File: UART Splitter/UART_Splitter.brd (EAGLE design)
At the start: 40.6 x 24.1 mm, 31 parts, among them IC1 ATTINY10, Q1 12mhz, U1 74HC4052

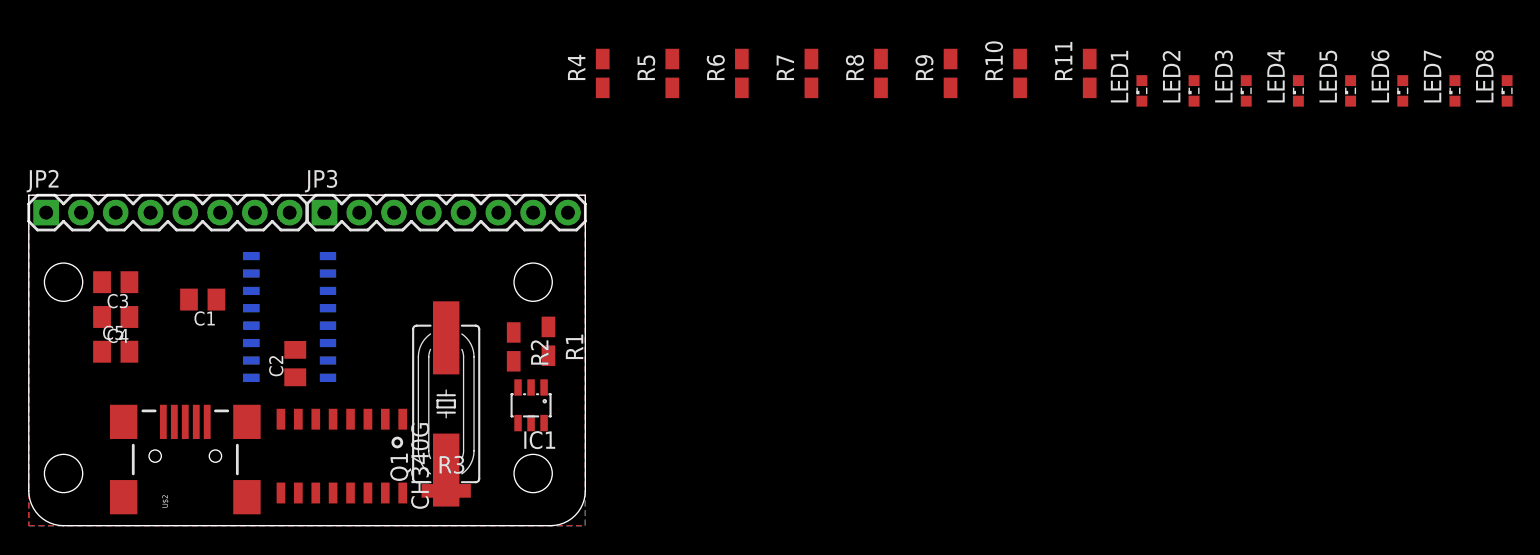
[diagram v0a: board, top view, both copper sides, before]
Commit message: UART Splitter
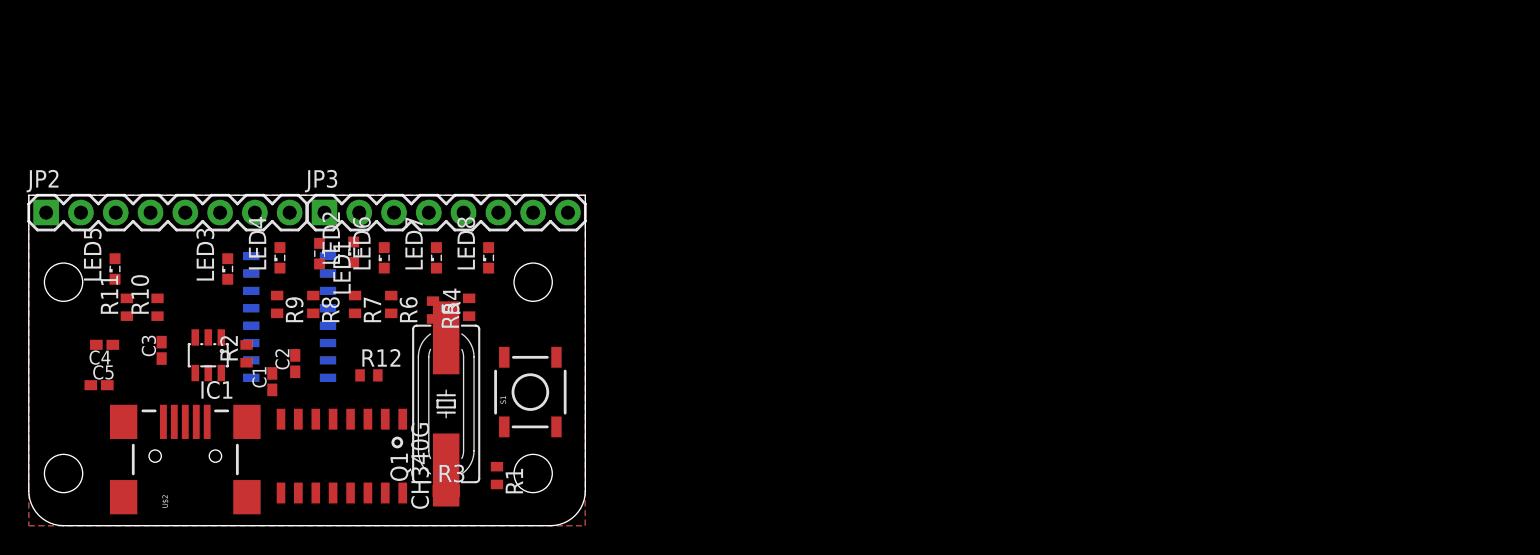
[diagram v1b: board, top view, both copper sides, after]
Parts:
- added R12: 10k, resistor:R0402
- added S1: (no value), SparkFun-Electromechanical:TACTILE_SWITCH_SMD
- C1, C2, C3, C4, C5: device resistor:C0805K -> resistor:C0402K
- R1, R10, R11, R2, R3, R4, R5, R6, R7, R8, R9: device resistor:R0805W -> resistor:R0402
- moved LED5 91.2 mm to (35.5, 18.7)
- moved LED3 75.5 mm to (43.7, 18.7)
- moved LED4 75.4 mm to (47.5, 19.6)
- moved LED6 75.4 mm to (55.2, 19.6)
- moved LED7 75.4 mm to (59.0, 19.6)
- moved LED8 75.4 mm to (62.8, 19.6)
- moved R11 72.3 mm to (36.4, 16.0)
- moved R10 65.3 mm to (38.6, 16.0)
- moved LED2 62.5 mm to (52.9, 20.0)
- moved LED1 61.2 mm to (50.4, 19.9), turned to 270 degrees
- moved R9 52.0 mm to (47.3, 16.2), turned to 270 degrees
- moved R8 44.8 mm to (50.0, 16.2), turned to 270 degrees
- moved R7 37.3 mm to (53.0, 16.2), turned to 270 degrees
- moved R6 30.7 mm to (55.7, 16.2), turned to 270 degrees
- moved R5 24.6 mm to (58.7, 15.7), turned to 270 degrees
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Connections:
- new net N$13: R12.1, U1.6
- net GND: now also S1.3, S1.4
- net N$2: now also R1.2
- net N$6: no longer R1.1
- net N$7: now also IC1.3, R1.1, S1.1, S1.2; no longer U1.6
- net N$8: now also IC1.6, R12.2; no longer IC1.1, R1.2
- net N$9: now also IC1.1; no longer IC1.3

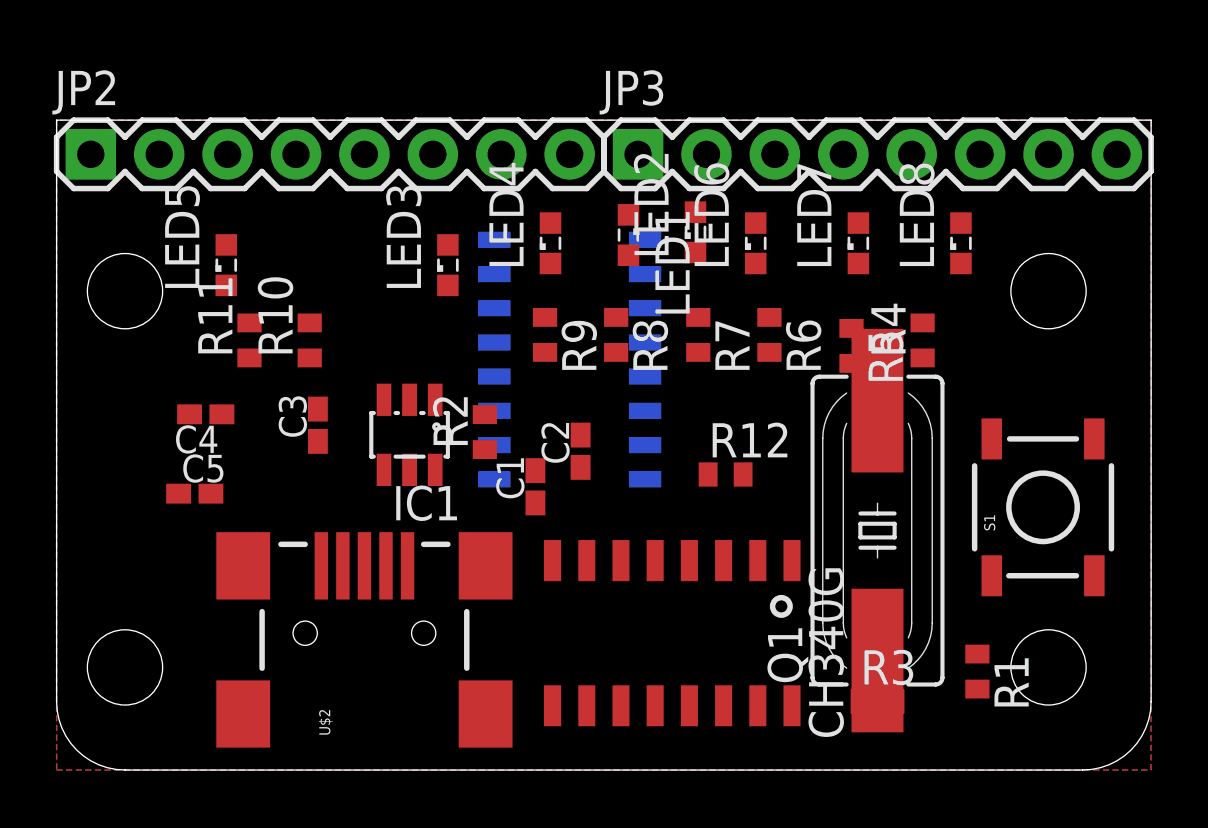
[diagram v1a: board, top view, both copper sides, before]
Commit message: UART Splitter
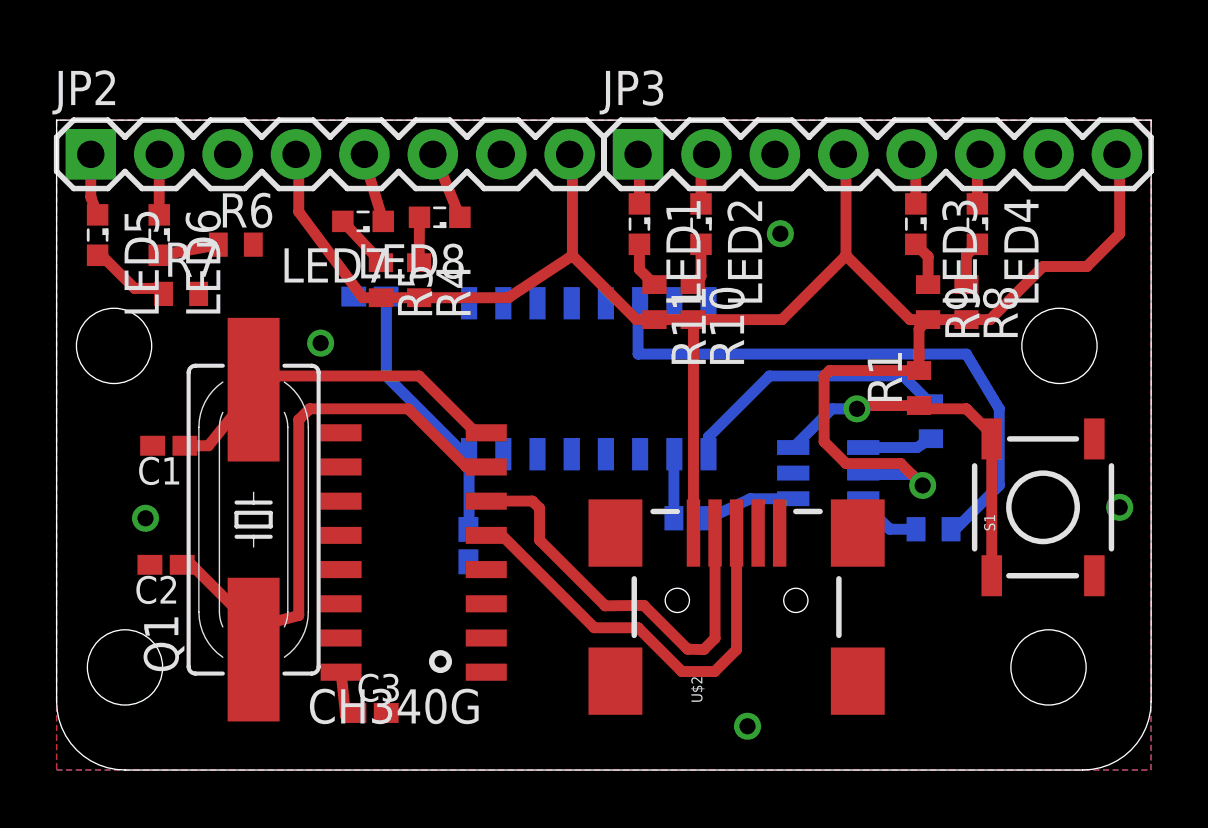
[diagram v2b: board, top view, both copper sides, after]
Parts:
- moved Q1 23.2 mm to (36.5, 9.30)
- moved LED6 22.2 mm to (33.0, 19.9), turned to 270 degrees
- moved R6 20.1 mm to (35.9, 19.5), turned to 0 degrees
- moved LED8 19.4 mm to (43.4, 20.5), turned to 180 degrees
- moved R7 19.3 mm to (33.8, 17.7), turned to 0 degrees
- moved R4 18.8 mm to (42.7, 18.2), turned to 270 degrees
- moved LED7 18.4 mm to (40.6, 20.4), turned to 180 degrees
- moved R5 17.6 mm to (41.2, 18.2)
- moved LED3 17.4 mm to (61.1, 20.3), turned to 270 degrees
- moved C2 16.0 mm to (33.3, 7.62), turned to 180 degrees
- moved LED4 15.9 mm to (63.4, 20.3), turned to 270 degrees
- moved IC1 15.6 mm to (57.9, 11.0), flipped to the bottom, turned to 90 degrees
- moved R11 15.1 mm to (51.4, 17.4), turned to 270 degrees
- moved R10 14.3 mm to (52.8, 17.4), turned to 270 degrees
- moved R9 14.3 mm to (61.6, 17.4)
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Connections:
- net N$14 renamed LED_TX3
- net N$15 renamed LED_RX3
- net N$16 renamed LED_TX2
- net N$17 renamed LED_RX2
- net N$18 renamed LED_TX1
- net N$19 renamed LED_RX1
- net N$20 renamed LED_TX0
- net N$21 renamed LED_RX0
- removed net N$1: U$1.1, U$2.GND
- removed net N$2: C3.1, C4.1, C5.1, IC1.5, R1.2, U$1.16, U$2.VBUS, U1.16
- net GND: now also U$1.1, U$2.GND
- net N$6: now also R3.1
- net RX1: now also LED3.C
- net RX2: now also LED5.C
- net RX3: now also LED7.C
- net TX0: now also LED2.C
- net TX1: now also LED4.C
- net TX2: now also LED6.C
- net TX3: now also LED8.C
- net VCC: now also C3.1, C4.1, C5.1, IC1.5, R1.2, U$1.16, U$2.VBUS, U1.16
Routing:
- net VCC: track 0.00 -> 84.3 mm, vias 0 -> 1
- net N$10: track 0.00 -> 22.1 mm
- net N$13: track 0.00 -> 21.8 mm
- net N$3: track 0.00 -> 16.1 mm
- net N$4: track 0.00 -> 15.6 mm
- net N$7: track 0.00 -> 13.7 mm, vias 0 -> 1
- net N$11: track 0.00 -> 13.2 mm
- net N$6: track 0.00 -> 10.3 mm
- net LED_RX2: track 0.00 -> 3.30 mm
- net N$9: track 0.00 -> 3.29 mm
- net RX3: track 0.00 -> 2.62 mm
- net N$12: track 0.00 -> 2.61 mm
- net TX3: track 0.00 -> 2.55 mm
- net N$8: track 0.00 -> 2.52 mm
- net N$5: track 0.00 -> 2.39 mm
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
